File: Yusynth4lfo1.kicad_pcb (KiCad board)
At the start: 2 copper layers, 91.9 x 110 mm, 72 parts, among them J1 Conn_01x13_Male, J2 Conn_01x13_Female, J3 Conn_02x05_Counter_Clockwise, J4 FM level, J5 270°, J6 180°, J7 0°, J8 90°, Q1 BC547C, Q2 BC557C, Q3 BC557C, Q4 BC547C, Q5 BC547C, Q6 BC547C, SW1 SW_Push_DPDT, U1 LM13700, U2 TL074, U3 TL074

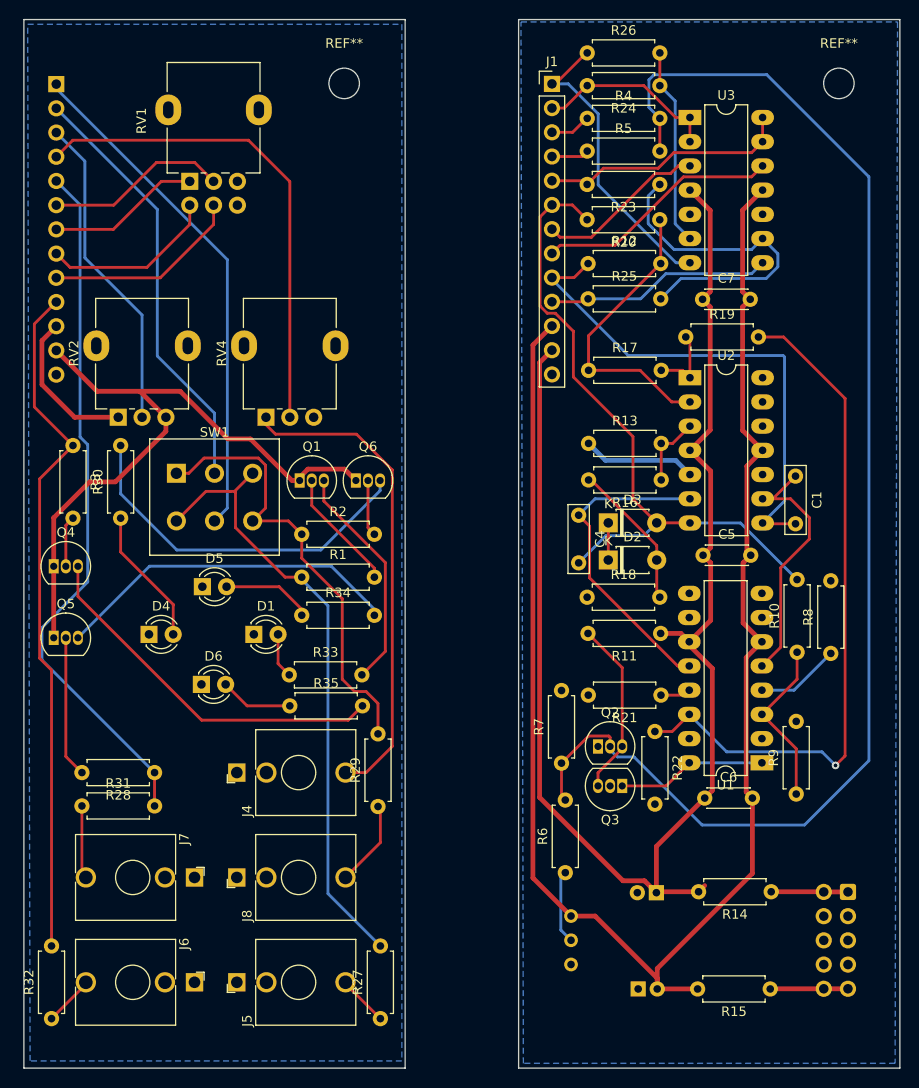
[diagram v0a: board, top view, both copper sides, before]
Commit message: nouvelle version
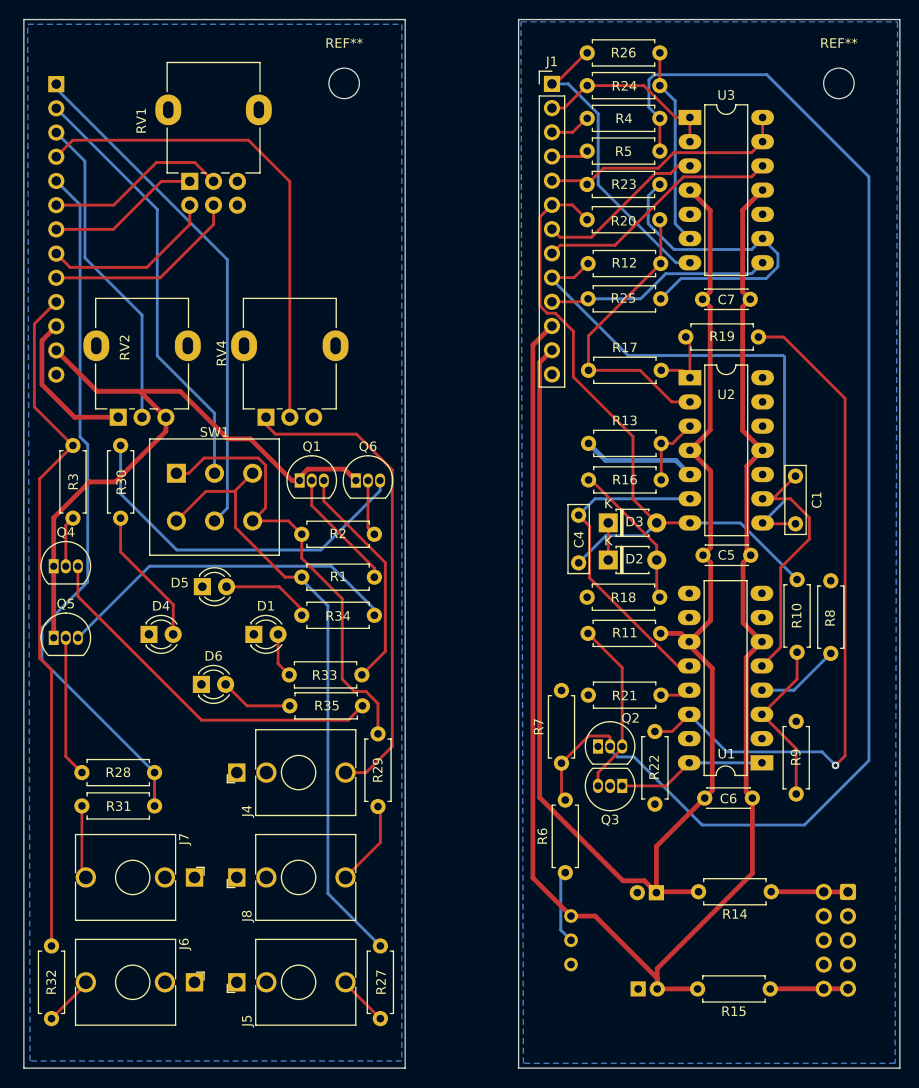
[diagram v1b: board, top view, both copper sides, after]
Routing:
- net +12V: track 226.4 -> 225.5 mm
